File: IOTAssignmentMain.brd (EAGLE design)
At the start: 196.4 x 163.8 mm, 7 parts, among them U1 ARDUINO-UNO-R3-SHIELD, U2 PINHD-1X08_1X08M

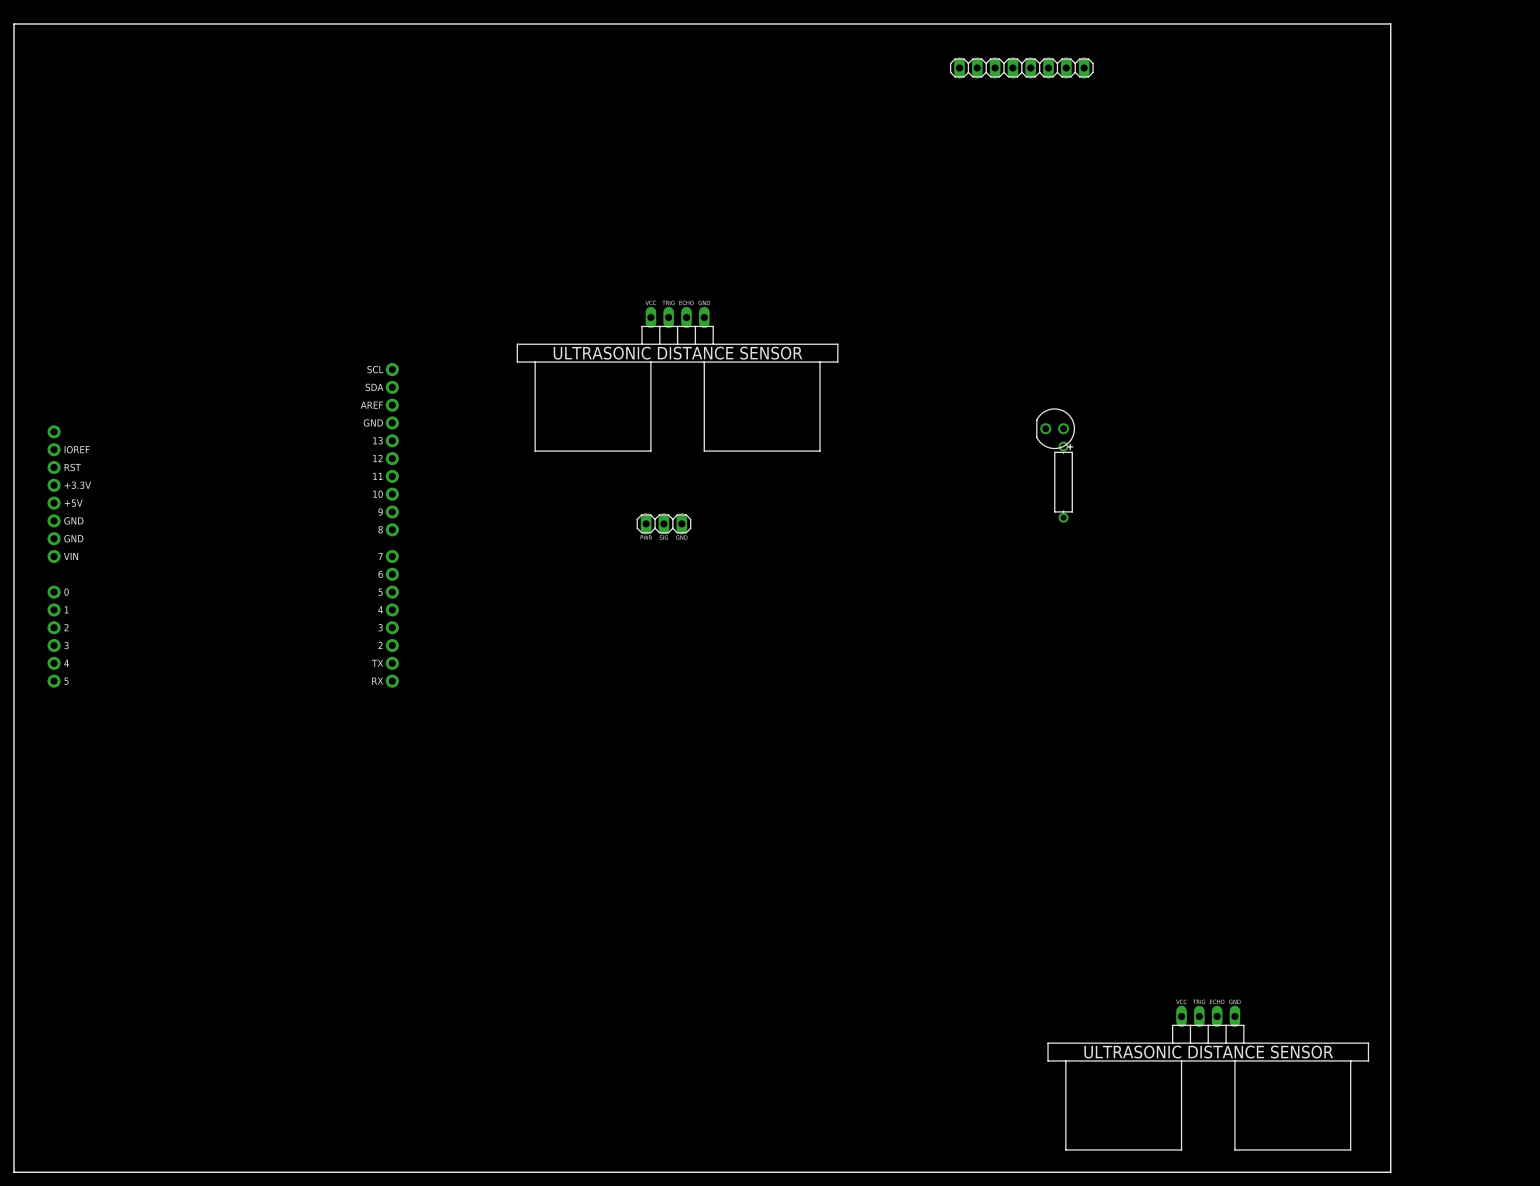
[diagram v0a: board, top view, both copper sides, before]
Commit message: new commit
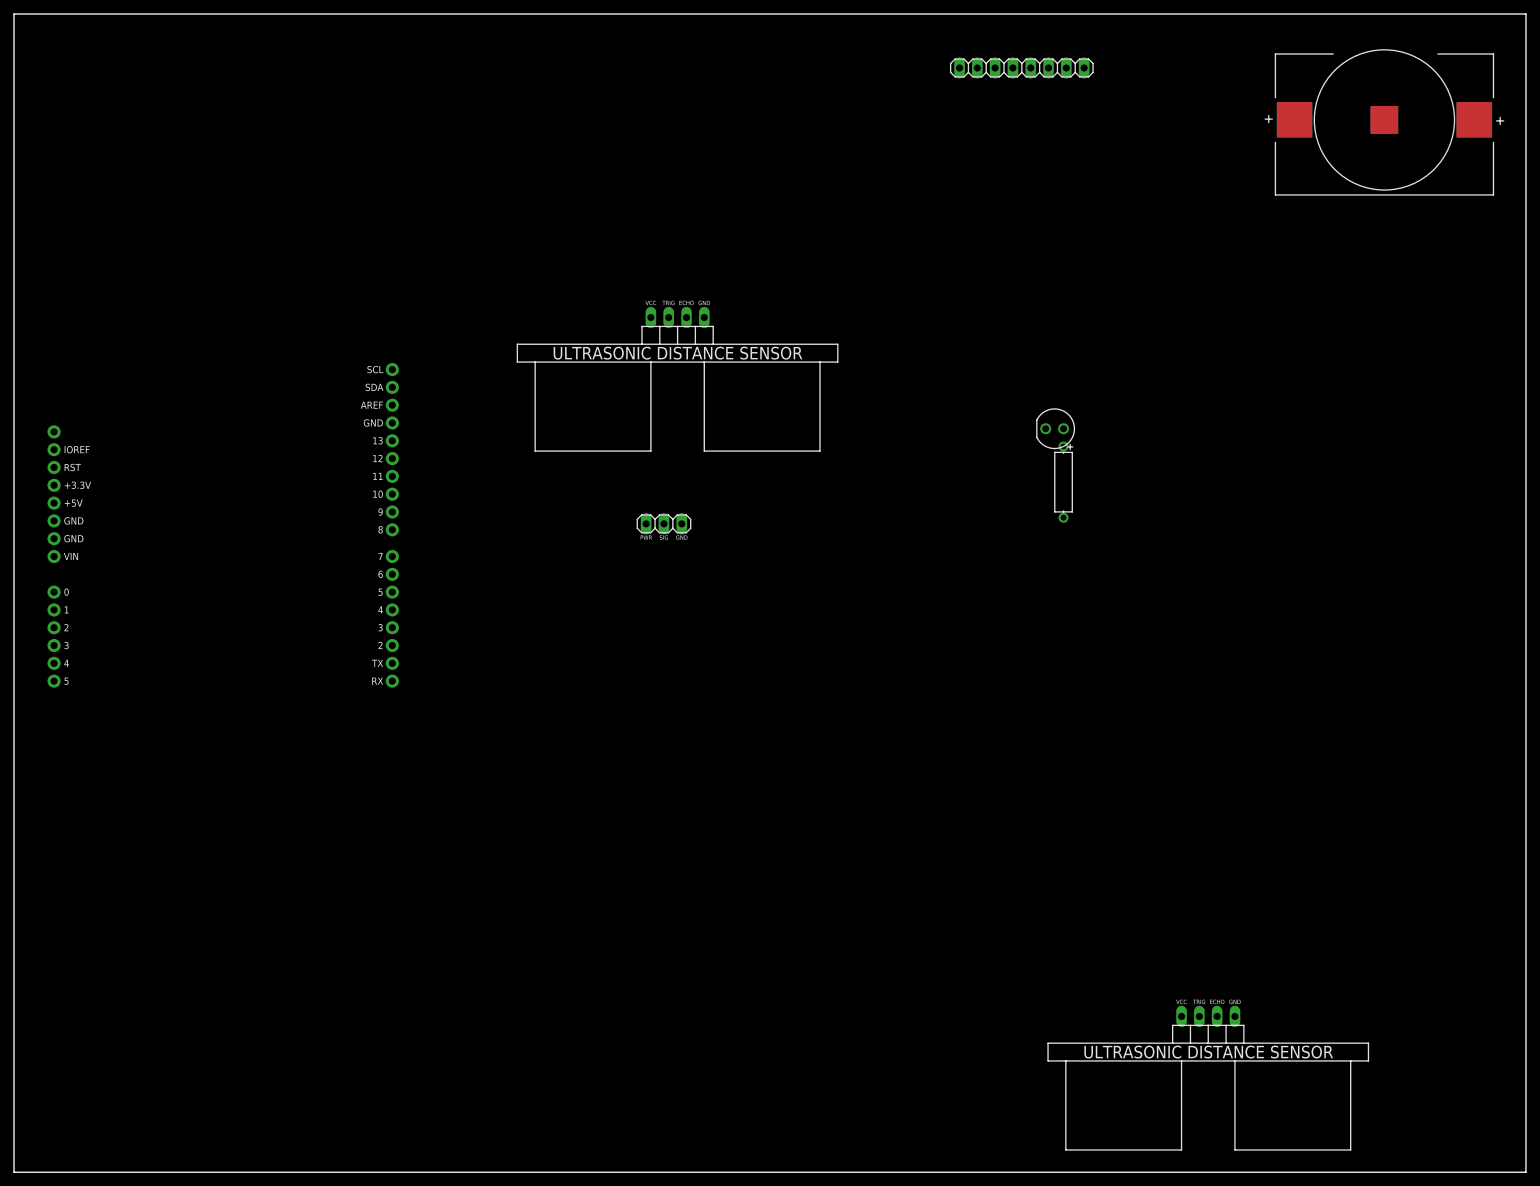
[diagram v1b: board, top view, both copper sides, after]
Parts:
- added BAT1: BR2016, Tinkercad:BAT_3002
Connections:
- new net BAT1+: BAT1.P, BAT1.P1, U2.1
- new net BAT1-: BAT1.N, U2.2
- net U1_5V: no longer U2.1
- net U1_GND: no longer U2.2
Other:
- board size 196.4 x 163.8 mm -> 215.7 x 165.2 mm
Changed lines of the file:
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@@
 <board>
 <plain>
-<wire x1="0" y1="0" x2="196.4208074543199" y2="0" width="0" layer="20"/>
-<wire x1="196.4208074543199" y1="0" x2="196.4208074543199" y2="163.82330842146052" width="0" layer="20"/>
-<wire x1="196.4208074543199" y1="163.82330842146052" x2="0" y2="163.82330842146052" width="0" layer="20"/>
-<wire x1="0" y1="163.82330842146052" x2="0" y2="0" width="0" layer="20"/>
+<wire x1="0" y1="0" x2="215.71588068697233" y2="0" width="0" layer="20"/>
+<wire x1="215.71588068697233" y1="0" x2="215.71588068697233" y2="165.24682651706956" width="0" layer="20"/>
+<wire x1="215.71588068697233" y1="165.24682651706956" x2="0" y2="165.24682651706956" width="0" layer="20"/>
+<wire x1="0" y1="165.24682651706956" x2="0" y2="0" width="0" layer="20"/>
 </plain>
 <attributes/>
@@
 <elements>
 <element name="SERVO1" library="Tinkercad" package="SM-S2309S" package3d_urn="urn:adsk.eagle:package:32659984/2" value="SERVOSM-S2309S" x="92.7307" y="92.507" smashed="yes"/>
+<element name="DIST2" library="Tinkercad" package="HC-SR04" package3d_urn="urn:adsk.eagle:package:32384643/2" value="DISTANCE-SENSOR-4PINHC-SR04" x="170.3858" y="22.225" smashed="yes"/>
 <element name="DIST1" library="Tinkercad" package="HC-SR04" package3d_urn="urn:adsk.eagle:package:32384643/2" value="DISTANCE-SENSOR-4PINHC-SR04" x="94.6732" y="121.9416" smashed="yes"/>
-<element name="U2" library="Tinkercad" package="1X08" package3d_urn="urn:adsk.eagle:package:22409/2" value="PINHD-1X08_1X08M" x="143.7887" y="157.5495" smashed="yes"/>
 <element name="U1" library="Tinkercad" package="ARDUINO-UNO-R3-SHIELD" package3d_urn="urn:adsk.eagle:package:32092383/4" value="ARDUINO-UNO-R3-SHIELD" x="29.845" y="95.4678" rot="R180" smashed="yes"/>
-<element name="DIST2" library="Tinkercad" package="HC-SR04" package3d_urn="urn:adsk.eagle:package:32384643/2" value="DISTANCE-SENSOR-4PINHC-SR04" x="170.3858" y="22.225" smashed="yes"/>
 <element name="R1" library="Tinkercad" package="RESAD1016W63L850D250B" package3d_urn="urn:adsk.eagle:package:31513020/2" value="1k" x="149.7382" y="98.4578" rot="R90" smashed="yes"/>
 <element name="D1" library="Tinkercad" package="LEDRD254W60D565H860B" package3d_urn="urn:adsk.eagle:package:16378508/2" value="RED" x="148.4682" y="106.0778" rot="R180" smashed="yes">
@@
 <attribute name="VALUE" value="LED_RED" x="148.4682" y="106.0778" size="1.778" layer="27" display="off"/>
 </element>
+<element name="U2" library="Tinkercad" package="1X08" package3d_urn="urn:adsk.eagle:package:22409/2" value="PINHD-1X08_1X08M" x="143.7887" y="157.5495" smashed="yes"/>
+<element name="BAT1" library="Tinkercad" package="BAT_3002" package3d_urn="urn:adsk.eagle:package:27510254/3" value="BR2016" x="195.5229" y="149.4868" rot="R360" smashed="yes">
+<attribute name="CATEGORY" value="Battery-Holder" x="195.5229" y="149.4868" size="1.778" layer="27" display="off"/>
+<attribute name="CELL_DIAMETER" value="20mm" x="195.5229" y="149.4868" size="1.778" layer="27" display="off"/>
+<attribute name="DESCRIPTION" value="Battery Retainer Coin, 20.0mm 1 Cell SMD (SMT) Tab" x="195.5229" y="149.4868" size="1.778" layer="27" display="off"/>
+<attribute name="MANUFACTURER" value="Keystone Electronics" x="195.5229" y="149.4868" size="1.778" layer="27" display="off"/>
+<attribute name="MPN" value="3002" x="195.5229" y="149.4868" size="1.778" layer="27" display="off"/>
+<attribute name="PART_STATUS" value="ACTIVE" x="195.5229" y="149.4868" size="1.778" layer="27" display="off"/>
+<attribute name="ROHS_COMPLIANT" value="COMPLIANT" x="195.5229" y="149.4868" size="1.778" layer="27" display="off"/>
+<attribute name="SERIES" value="-" x="195.5229" y="149.4868" size="1.778" layer="27" display="off"/>
+<attribute name="SUB_CATEGORY" value="Holder" x="195.5229" y="149.4868" size="1.778" layer="27" display="off"/>
+<attribute name="TYPE" value="Coin Cell" x="195.5229" y="149.4868" size="1.778" layer="27" display="off"/>
+<attribute name="VALUE" value="BR2016" x="195.5229" y="149.4868" size="1.778" layer="27" display="off"/>
+</element>
 </elements>
 <signals>
@@
 <contactref element="SERVO1" pad="3"/>
 <contactref element="DIST2" pad="4"/>
-<contactref element="U2" pad="2"/>
 <wire x1="5.715" y1="92.9278" x2="5.715" y2="90.3878" width="0" layer="19" extent="1-1"/>
 <wire x1="5.715" y1="92.9278" x2="53.975" y2="106.8978" width="0" layer="19" extent="1-1"/>
@@
 <wire x1="98.4832" y1="121.9416" x2="95.2707" y2="92.507" width="0" layer="19" extent="1-1"/>
 <wire x1="147.1982" y1="106.0778" x2="98.4832" y2="121.9416" width="0" layer="19" extent="1-1"/>
-<wire x1="147.1982" y1="106.0778" x2="137.4387" y2="157.5495" width="0" layer="19" extent="1-1"/>
 <wire x1="147.1982" y1="106.0778" x2="174.1958" y2="22.225" width="0" layer="19" extent="1-1"/>
 </signal>
@@
 <contactref element="SERVO1" pad="1"/>
 <contactref element="DIST2" pad="1"/>
-<contactref element="U2" pad="1"/>
 <wire x1="90.8632" y1="121.9416" x2="90.1907" y2="92.507" width="0" layer="19" extent="1-1"/>
-<wire x1="90.8632" y1="121.9416" x2="134.8987" y2="157.5495" width="0" layer="19" extent="1-1"/>
 <wire x1="5.715" y1="95.4678" x2="90.1907" y2="92.507" width="0" layer="19" extent="1-1"/>
 <wire x1="90.1907" y1="92.507" x2="166.5758" y2="22.225" width="0" layer="19" extent="1-1"/>
+</signal>
+<signal name="U1_D7">
+<contactref element="DIST2" pad="3"/>
+<contactref element="U1" pad="D7"/>
+<wire x1="171.6558" y1="22.225" x2="53.975" y2="87.8478" width="0" layer="19" extent="1-1"/>
+</signal>
+<signal name="U1_D6">
+<contactref element="DIST2" pad="2"/>
+<contactref element="U1" pad="D6"/>
+<wire x1="169.1158" y1="22.225" x2="53.975" y2="85.3078" width="0" layer="19" extent="1-1"/>
 </signal>
 <signal name="U1_D4">
@@
 <wire x1="93.4032" y1="121.9416" x2="53.975" y2="82.7678" width="0" layer="19" extent="1-1"/>
 </signal>
+<signal name="U1_D8">
+<contactref element="R1" pad="1"/>
+<contactref element="U1" pad="D8"/>
+<wire x1="149.7382" y1="93.3778" x2="53.975" y2="91.6578" width="0" layer="19" extent="1-1"/>
+</signal>
 <signal name="U2_8">
 <contactref element="U2" pad="8"/>
@@
 <wire x1="139.9787" y1="157.5495" x2="53.975" y2="70.0678" width="0" layer="19" extent="1-1"/>
 </signal>
-<signal name="U1_D8">
-<contactref element="R1" pad="1"/>
-<contactref element="U1" pad="D8"/>
-<wire x1="149.7382" y1="93.3778" x2="53.975" y2="91.6578" width="0" layer="19" extent="1-1"/>
-</signal>
-<signal name="U1_D7">
-<contactref element="DIST2" pad="3"/>
-<contactref element="U1" pad="D7"/>
-<wire x1="171.6558" y1="22.225" x2="53.975" y2="87.8478" width="0" layer="19" extent="1-1"/>
-</signal>
-<signal name="U1_D6">
-<contactref element="DIST2" pad="2"/>
-<contactref element="U1" pad="D6"/>
-<wire x1="169.1158" y1="22.225" x2="53.975" y2="85.3078" width="0" layer="19" extent="1-1"/>
-</signal>
 <signal name="D1_A">
 <contactref element="D1" pad="1"/>
@@
 <wire x1="149.7382" y1="106.0778" x2="149.7382" y2="103.5378" width="0" layer="19" extent="1-1"/>
 </signal>
+<signal name="BAT1-">
+<contactref element="BAT1" pad="N"/>
+<contactref element="U2" pad="2"/>
+<wire x1="195.5229" y1="150.1368" x2="137.4387" y2="157.5495" width="0" layer="19" extent="1-1"/>
+</signal>
+<signal name="BAT1+">
+<contactref element="BAT1" pad="P1"/>
+<contactref element="BAT1" pad="P"/>
+<contactref element="U2" pad="1"/>
+<wire x1="182.6979" y1="150.1368" x2="208.3479" y2="150.1368" width="0" layer="19" extent="1-1"/>
+<wire x1="182.6979" y1="150.1368" x2="134.8987" y2="157.5495" width="0" layer="19" extent="1-1"/>
+</signal>
 </signals>
